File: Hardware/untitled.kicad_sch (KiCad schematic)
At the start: 15 parts, among them IC1 LM74502HDDFR, J3 CarLVPowerConnector, Q12 PSMN8R5-40MSDX

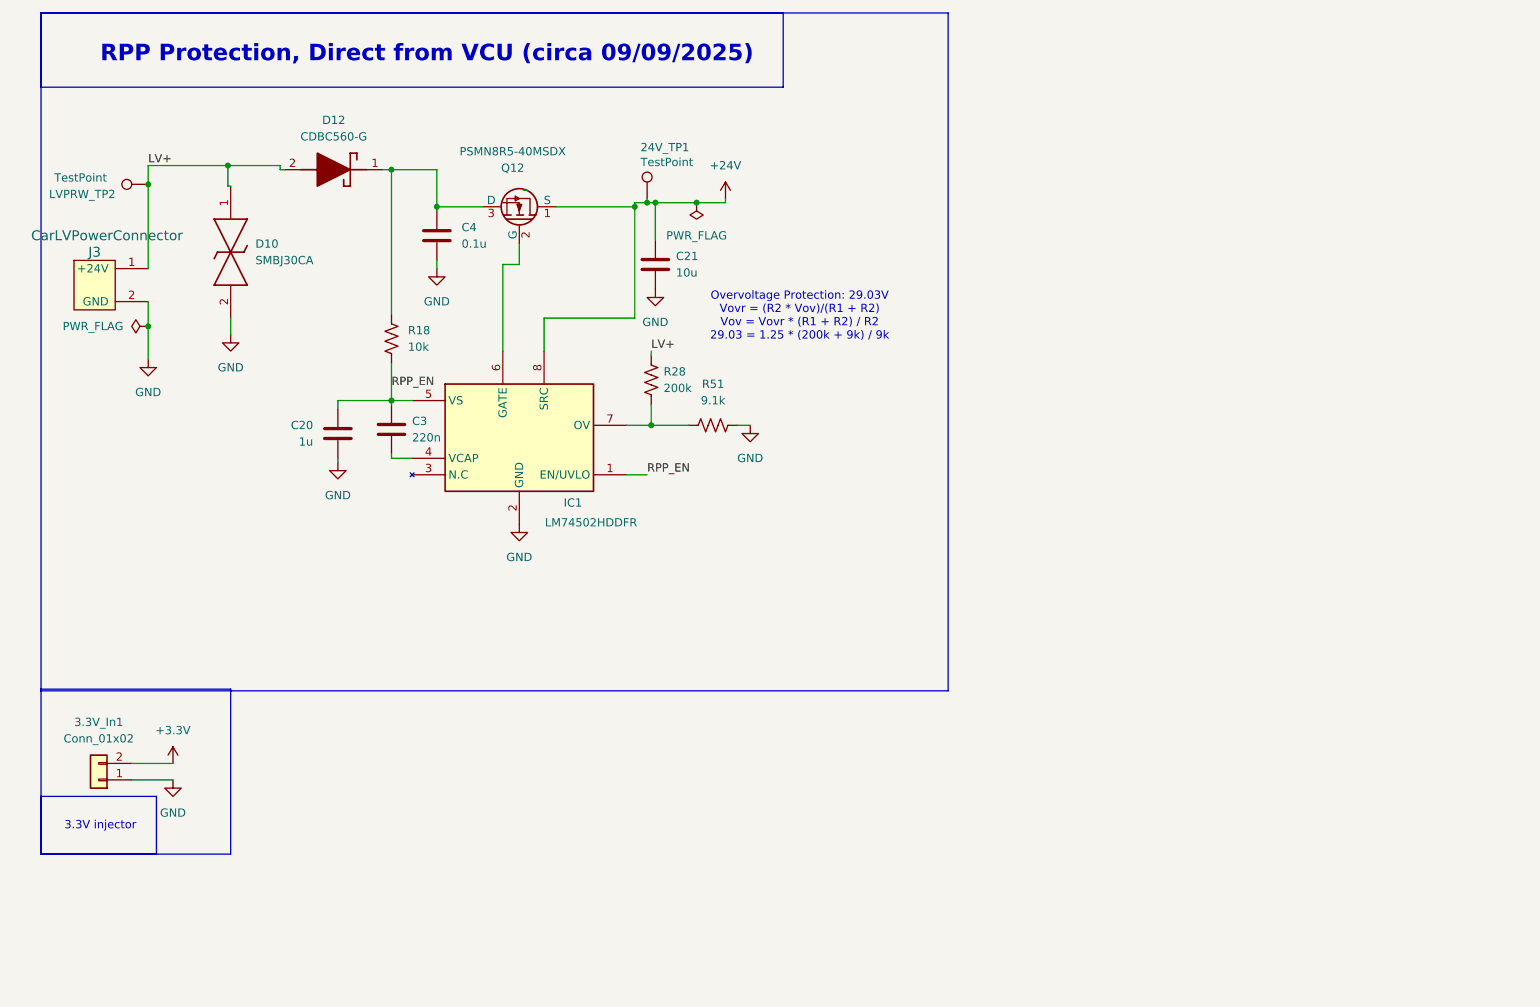
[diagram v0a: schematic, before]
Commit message: revB updates
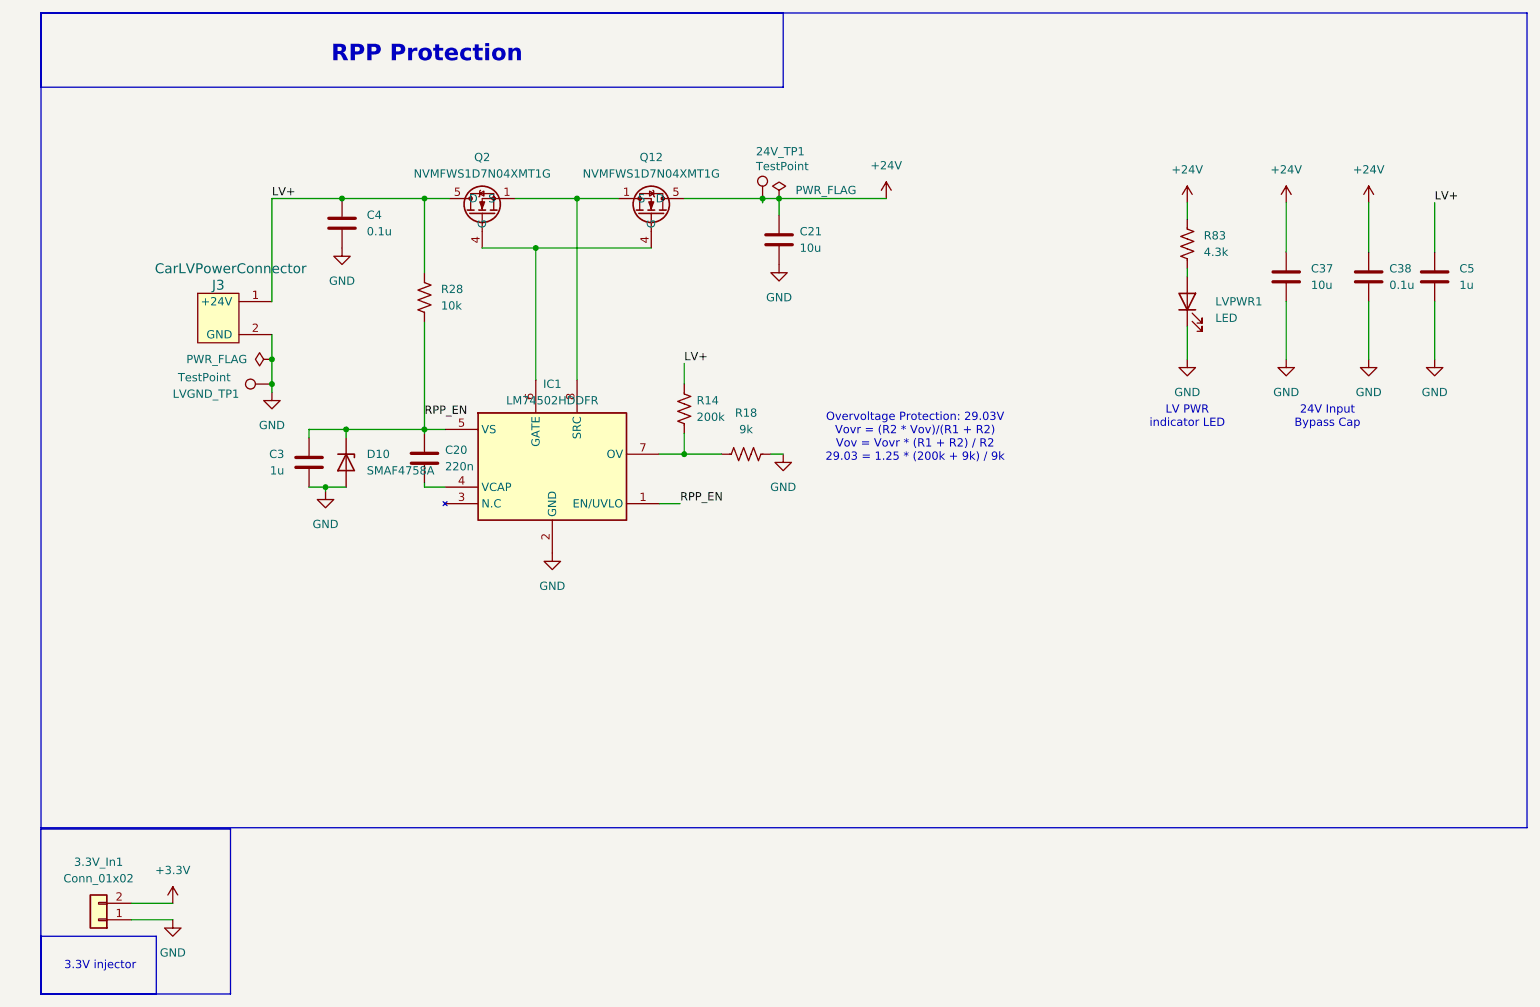
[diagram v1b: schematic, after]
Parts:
- removed D10: SMBJ30CA, DIOM5436X244N, symbol TVS Diode:SMBJ30CA
- removed D12: CDBC560-G, Schlotty:DIOM7959X262N, symbol Schott:CDBC560-G
- removed LVPRW_TP2: TestPoint, TestPoint:TestPoint_Pad_1.0x1.0mm, symbol Connector:TestPoint
- removed Q12: PSMN8R5-40MSDX, UTSVT_Power:PSMN8R5-40MSDX, symbol utsvt_power:PSMN8R5-40MSDX
- removed R28: 200k, Resistor_SMD:R_0603_1608Metric, symbol Device:R_US
- removed R51: 9.1k, Resistor_SMD:R_0603_1608Metric, symbol Device:R_US
- added C37: 10u, Capacitor_SMD:C_0805_2012Metric_Pad1.18x1.45mm_HandSolder, symbol Device:C
- added C38: 0.1u, Capacitor_SMD:C_0603_1608Metric_Pad1.08x0.95mm_HandSolder, symbol Device:C
- added C5: 1u, Capacitor_SMD:C_0603_1608Metric_Pad1.08x0.95mm_HandSolder, symbol Device:C
- added D10: SMAF4758A, UTSVT_Passives:SODFL5026X125N, symbol Device:D_Zener
- added LVGND_TP1: TestPoint, TestPoint:TestPoint_Pad_2.0x2.0mm, symbol Connector:TestPoint
- added LVPWR1: LED, LED_SMD:LED_0603_1608Metric_Pad1.05x0.95mm_HandSolder, symbol Device:LED
- added Q12, Q2: NVMFWS1D7N04XMT1G, UTSVT_Power:NVMFWS3D0P04M8LT1G, symbol UTSVT_Power:NVMFWS1D7N04XMT1G
- added R14: 200k, Resistor_SMD:R_0603_1608Metric_Pad0.98x0.95mm_HandSolder, symbol Device:R_US
- added R18: 9k, Resistor_SMD:R_0603_1608Metric_Pad0.98x0.95mm_HandSolder, symbol Device:R_US
- added R83: 4.3k, Resistor_SMD:R_0603_1608Metric_Pad0.98x0.95mm_HandSolder, symbol Device:R_US
- 24V_TP1: footprint TestPoint:TestPoint_Pad_1.0x1.0mm -> TestPoint:TestPoint_Pad_2.0x2.0mm
- C20: value 1u -> 220n; footprint Capacitor_SMD:C_0603_1608Metric -> Capacitor_SMD:C_0603_1608Metric_Pad1.08x0.95mm_HandSolder; Manufactuerer TAIYO YUDEN -> (none); Mouser Part Number (none) -> 963-MSASU168SB7224KT; P/N MLASU168SB5105KTNA01 -> MSASU168SB7224KTNB25
- C21: footprint Capacitor_SMD:C_0805_2012Metric -> Capacitor_SMD:C_0805_2012Metric_Pad1.18x1.45mm_HandSolder; Manufactuerer Murata Electronics -> (none); Mouser Part Number (none) -> 81-GRM21BR61H106KE3K
- C3: value 220n -> 1u; footprint Capacitor_SMD:C_0603_1608Metric -> Capacitor_SMD:C_0603_1608Metric_Pad1.08x0.95mm_HandSolder; Manufactuerer TAIYO YUDEN -> (none); Mouser Part Number (none) -> 963-UMK107BJ105KA-T; P/N MSASU168SB7224KTNB25 -> UMK107BJ105KA-T
- C4: Manufactuerer TAIYO YUDEN -> (none); Mouser Part Number (none) -> 963-HMK107B7104KA-T; P/N MLASH168SB7104KTNA01 -> HMK107B7104KA-T
- IC1: Manufactuerer Texas Instruments -> (none); Manufacturer_Part_Number (none) -> LM74502HDDFR
- J3: Manufactuerer Molex -> (none); Mouser Part Number (none) -> 538-105309-1102; P/N 105309-1102 -> 105309-1102
- R28: renamed from R18; footprint Resistor_SMD:R_0603_1608Metric -> Resistor_SMD:R_0603_1608Metric_Pad0.98x0.95mm_HandSolder; Manufactuerer Vishay -> (none); Mouser Part Number (none) -> 71-CRCW060310K0FKEI; P/N CRCW060310K0FKEI -> CRCW060310K0FKEI
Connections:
- net +24V: now also C37.1, C38.1, Q12.5 (D), Q12.6 (D), Q12.7 (D), Q12.8 (D), Q12.9 (D), R83.1; no longer IC1.8 (SRC)
- net GND: now also C3.1, C4.2, C37.2, C38.2, C5.2, D10.2 (A), LVGND_TP1.1, LVPWR1.1 (K), R18.2; no longer C20.1, C4.1
- net LV+: now also C4.1, R28.1, C5.1, Q2.5 (D), Q2.6 (D), Q2.7 (D), Q2.8 (D), Q2.9 (D), R14.1
- net RPP_EN: now also C20.1, C3.2, D10.1 (K); no longer C20.2, C3.1
- net at IC1.4 (VCAP): now also C20.2; no longer C3.2
- net at IC1.6 (GATE): now also Q12.4 (G), Q2.4 (G)
- net at IC1.7 (OV): now also R14.2, R18.1
- new net: IC1.8 (SRC), Q12.1 (S), Q12.2 (S), Q12.3 (S), Q2.1 (S), Q2.2 (S), Q2.3 (S)
- new net: LVPWR1.2 (A), R83.2
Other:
- note added: "24V Input Bypass Cap"
- note added: "LV PWR indicator LED"
- note added: "RPP Protection"
- note removed: "RPP Protection, Direct from VCU (circa 09/09/2025)"
- moved on the sheet: 24V_TP1, 3.3V_In1, IC1, R28
